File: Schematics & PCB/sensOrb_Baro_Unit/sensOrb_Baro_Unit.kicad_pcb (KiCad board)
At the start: 2 copper layers, 25.5 x 17 mm, 7 parts, among them J11 Conn_01x04, U1 MS583730BA01-50

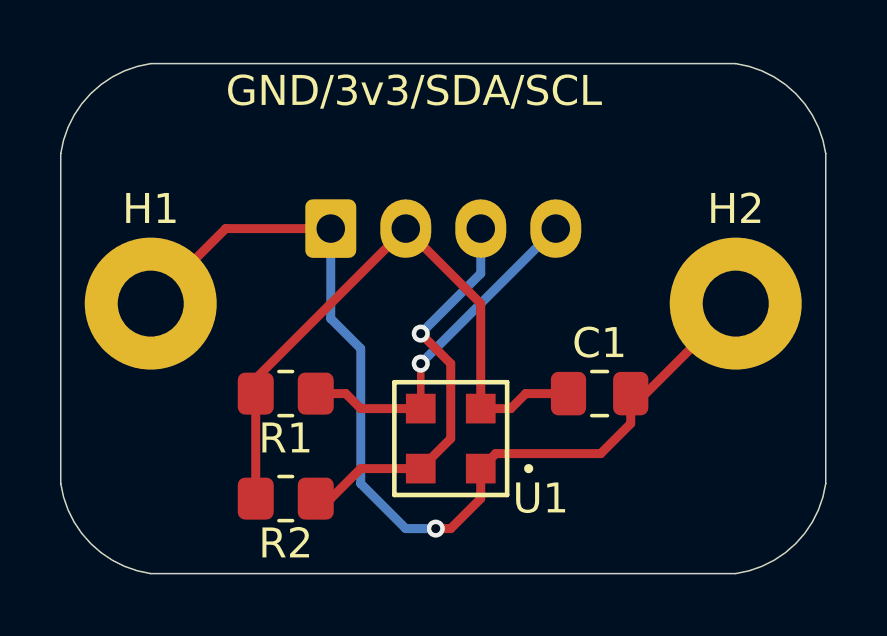
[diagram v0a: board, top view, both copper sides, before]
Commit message: Output Files Made
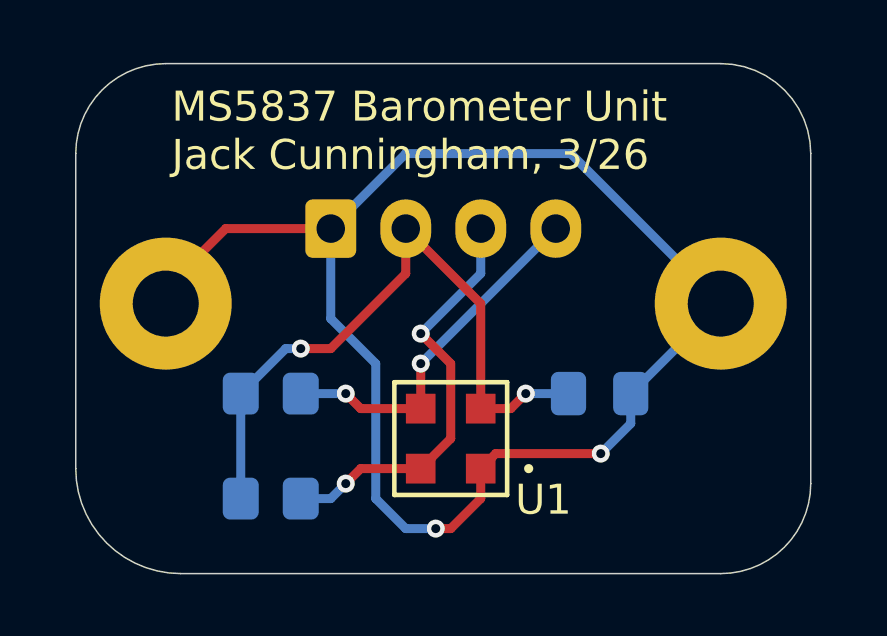
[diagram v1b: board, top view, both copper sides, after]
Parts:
- C1, R1, R2: moved to B.Cu
- moved H1 0.50 mm to (138.0, 102.0)
- moved H2 0.50 mm to (156.5, 102.0)
- moved R1 0.50 mm to (141.5, 105.0)
- moved R2 0.50 mm to (141.5, 108.5)
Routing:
- net GND: track 33.3 -> 49.2 mm, vias 1 -> 2
- net +3.3V: track 21.2 -> 22.3 mm, vias 0 -> 2
- net /SD0: track 13.6 -> 14.1 mm, vias 1 -> 2
- net /SC0: track 11.6 -> 12.1 mm, vias 1 -> 2
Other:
- board size 25.5 x 17 mm -> 24.5 x 17 mm
